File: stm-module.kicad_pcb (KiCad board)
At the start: 2 copper layers, 21 parts, among them J1 SWD, SW1 Reset, U1 STM32G474RETx, U2 TPS7A20xxxDBV, Y1 Crystal

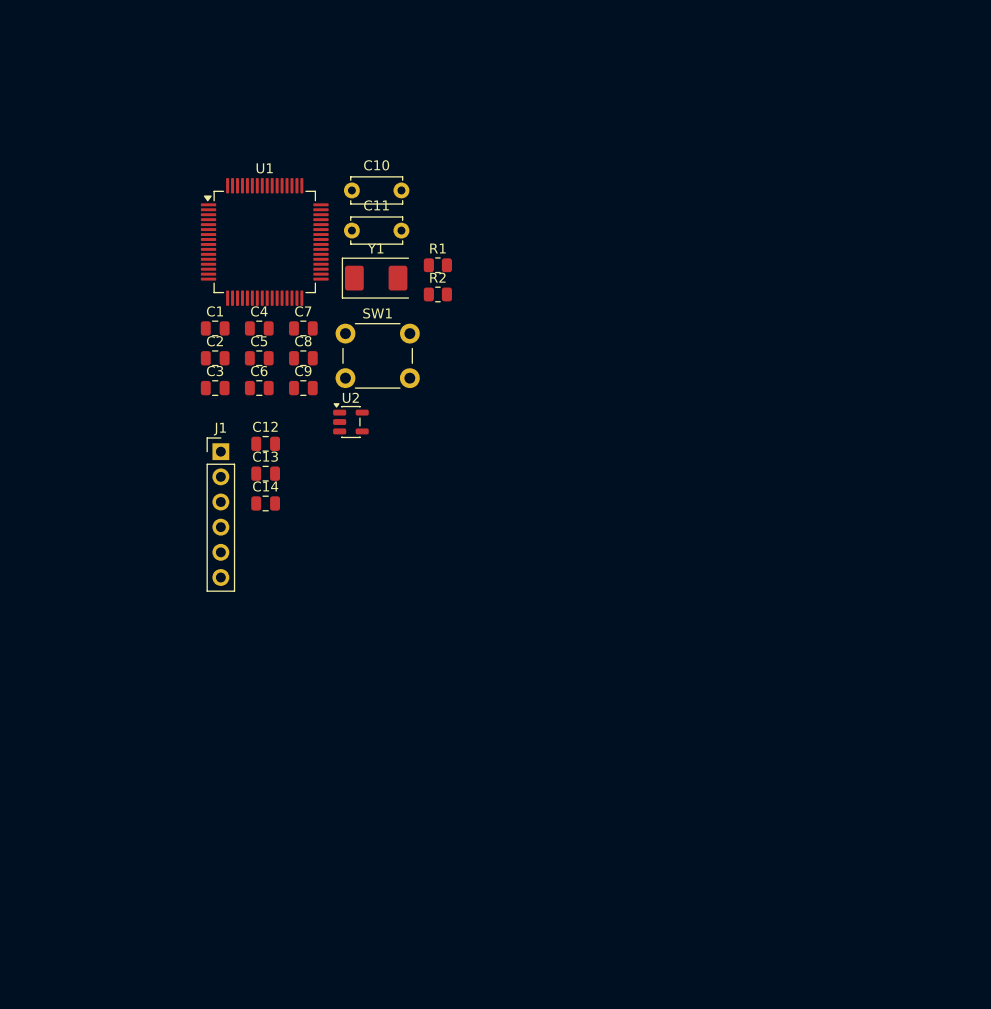
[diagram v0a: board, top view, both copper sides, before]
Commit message: pcb work
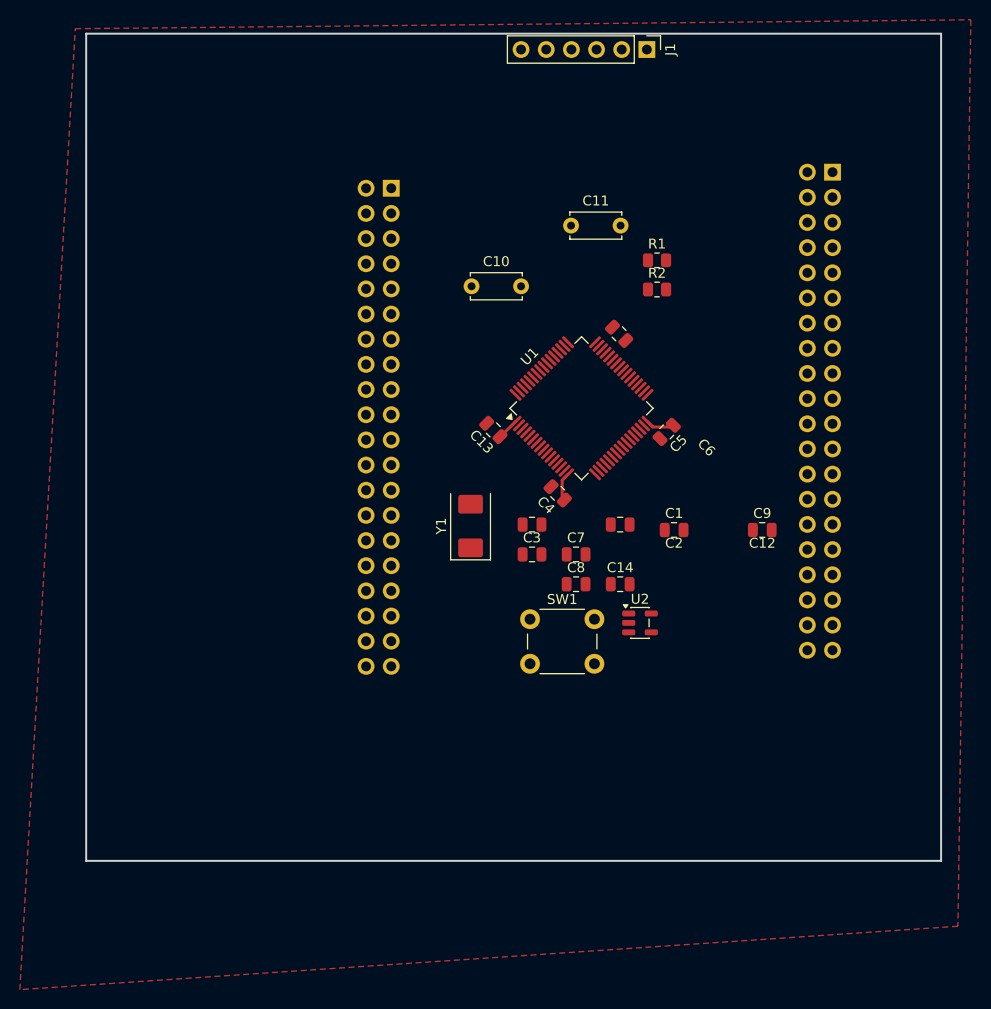
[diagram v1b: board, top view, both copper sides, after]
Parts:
- added J2: connectorL, Connector_PinHeader_2.54mm:PinHeader_2x20_P2.54mm_Vertical, B.Cu at (140.5, 85.3)
- added J3: connectorR, Connector_PinHeader_2.54mm:PinHeader_2x20_P2.54mm_Vertical, B.Cu at (185.0, 83.7)
- moved J1 59.1 mm to (166.3, 71.3), turned to -90 degrees
- moved C1 50.6 mm to (169.1, 119.8)
- moved C9 48.5 mm to (177.9, 119.8)
- moved C5 41.8 mm to (168.3, 109.9), turned to -135 degrees
- moved C6 36.7 mm to (163.5, 100.0), turned to -45 degrees
- moved C12 36.7 mm to (163.6, 119.3)
- moved C14 36.7 mm to (163.6, 125.3)
- moved C3 36.1 mm to (154.7, 122.3)
- moved U1 36.1 mm to (159.7, 107.5), turned to 45 degrees
- moved C2 36.1 mm to (154.7, 119.3)
- moved C7 35.8 mm to (159.2, 122.3)
- moved C8 35.8 mm to (159.2, 125.3)
- moved U2 35.5 mm to (165.6, 129.2)
- moved C4 34.4 mm to (157.3, 116.1), turned to 135 degrees
- moved SW1 34.3 mm to (154.5, 128.8)
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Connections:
- net /3.3V renamed +3.3V
- net /5V renamed +5V
- net /GND renamed GND
- net Net-(J1-Pin_3) renamed /PA13
- net Net-(J1-Pin_4) renamed /PA14
- net Net-(J1-Pin_6) renamed /PB3
- net Net-(U1-PB8) renamed /PB8
- U1 pad 10: unconnected-(U1-PC2-Pad10) -> /PC2
- U1 pad 11: unconnected-(U1-PC3-Pad11) -> /PC3
- U1 pad 12: unconnected-(U1-PA0-Pad12) -> /PA0
- U1 pad 13: unconnected-(U1-PA1-Pad13) -> /PA1
- U1 pad 14: unconnected-(U1-PA2-Pad14) -> /PA2
- U1 pad 17: unconnected-(U1-PA3-Pad17) -> /PA3
- U1 pad 18: unconnected-(U1-PA4-Pad18) -> /PA4
- U1 pad 19: unconnected-(U1-PA5-Pad19) -> /PA5
- U1 pad 2: unconnected-(U1-PC13-Pad2) -> /PC13
- U1 pad 20: unconnected-(U1-PA6-Pad20) -> /PA6
- U1 pad 21: unconnected-(U1-PA7-Pad21) -> /PA7
- U1 pad 22: unconnected-(U1-PC4-Pad22) -> /PC4
- U1 pad 23: unconnected-(U1-PC5-Pad23) -> /PC5
- U1 pad 24: unconnected-(U1-PB0-Pad24) -> /PB0
- U1 pad 25: unconnected-(U1-PB1-Pad25) -> /PB1
- U1 pad 26: unconnected-(U1-PB2-Pad26) -> /PB2
- U1 pad 3: unconnected-(U1-PC14-Pad3) -> /PC14
- U1 pad 30: unconnected-(U1-PB10-Pad30) -> /PB10
- U1 pad 33: unconnected-(U1-PB11-Pad33) -> /PB11
- U1 pad 34: unconnected-(U1-PB12-Pad34) -> /PB12
- U1 pad 35: unconnected-(U1-PB13-Pad35) -> /PB13
- U1 pad 36: unconnected-(U1-PB14-Pad36) -> /PB14
- U1 pad 37: unconnected-(U1-PB15-Pad37) -> /PB15
- U1 pad 38: unconnected-(U1-PC6-Pad38) -> /PC6
- U1 pad 39: unconnected-(U1-PC7-Pad39) -> /PC7
- U1 pad 4: unconnected-(U1-PC15-Pad4) -> /PC15
- U1 pad 40: unconnected-(U1-PC8-Pad40) -> /PC8
- U1 pad 41: unconnected-(U1-PC9-Pad41) -> /PC9
- U1 pad 42: unconnected-(U1-PA8-Pad42) -> /PA8
- U1 pad 43: unconnected-(U1-PA9-Pad43) -> /PA9
- U1 pad 44: unconnected-(U1-PA10-Pad44) -> /PA10
- U1 pad 45: unconnected-(U1-PA11-Pad45) -> /PA11
- U1 pad 46: unconnected-(U1-PA12-Pad46) -> /PA12
- U1 pad 51: unconnected-(U1-PA15-Pad51) -> /PA15
- U1 pad 52: unconnected-(U1-PC10-Pad52) -> /PC10
- U1 pad 53: unconnected-(U1-PC11-Pad53) -> /PC11
- U1 pad 54: unconnected-(U1-PC12-Pad54) -> /PC12
- U1 pad 55: unconnected-(U1-PD2-Pad55) -> /PD2
- U1 pad 57: unconnected-(U1-PB4-Pad57) -> /PB4
- U1 pad 58: unconnected-(U1-PB5-Pad58) -> /PB5
- U1 pad 59: unconnected-(U1-PB6-Pad59) -> /PB6
- U1 pad 60: unconnected-(U1-PB7-Pad60) -> /PB7
- U1 pad 62: unconnected-(U1-PB9-Pad62) -> /PB9
- U1 pad 8: unconnected-(U1-PC0-Pad8) -> /PC0
- U1 pad 9: unconnected-(U1-PC1-Pad9) -> /PC1
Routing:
- net +3.3V: track 0.00 -> 7.98 mm
- added copper zone on F.Cu, net GND
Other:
- board outline added: 86.3 x 83.5 mm
